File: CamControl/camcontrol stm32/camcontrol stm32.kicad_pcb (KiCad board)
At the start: 4 copper layers, 15.9 x 25.4 mm, 53 parts, among them J1 Power 1, J3 Power 1, J4 Power 1, J5 Conn_01x06, J6 Conn_01x02, J7 Power 1, J8 DNP, Q1 AO3401A, Q3 AO3401A, U1 BGS12WN6E6327, U2 BALFHB-WL-02D3, U3 STM32WLE4CCUx, U4 XC6206P332MR, U5 TPS25970LRPWR, U6 TPS25970LRPWR, U7 INA2180, Y1 32MHz

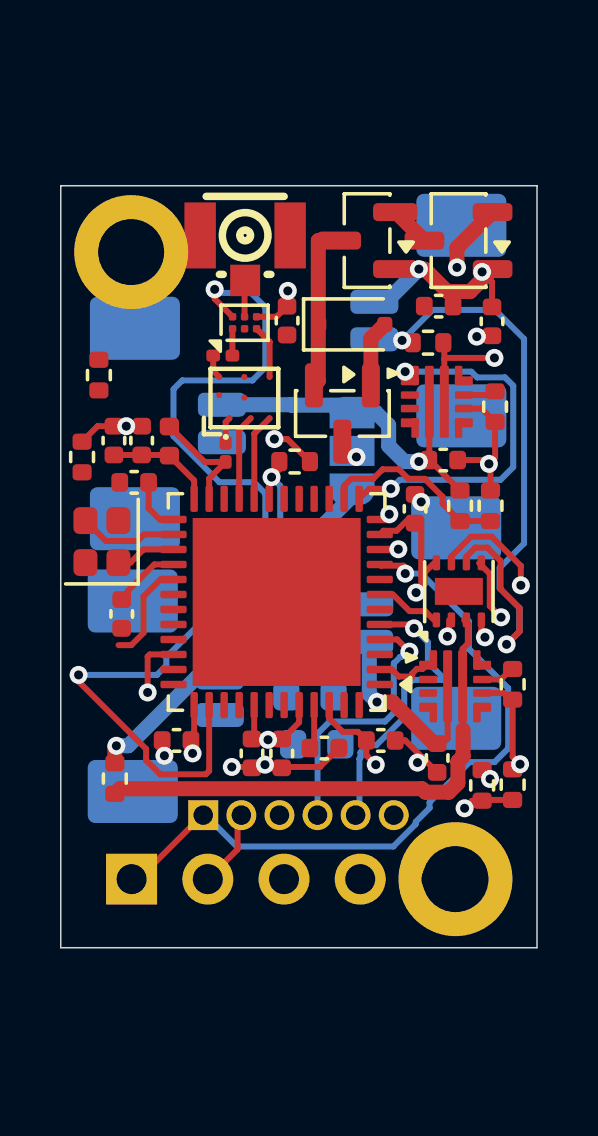
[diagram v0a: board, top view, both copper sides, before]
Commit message: final version?
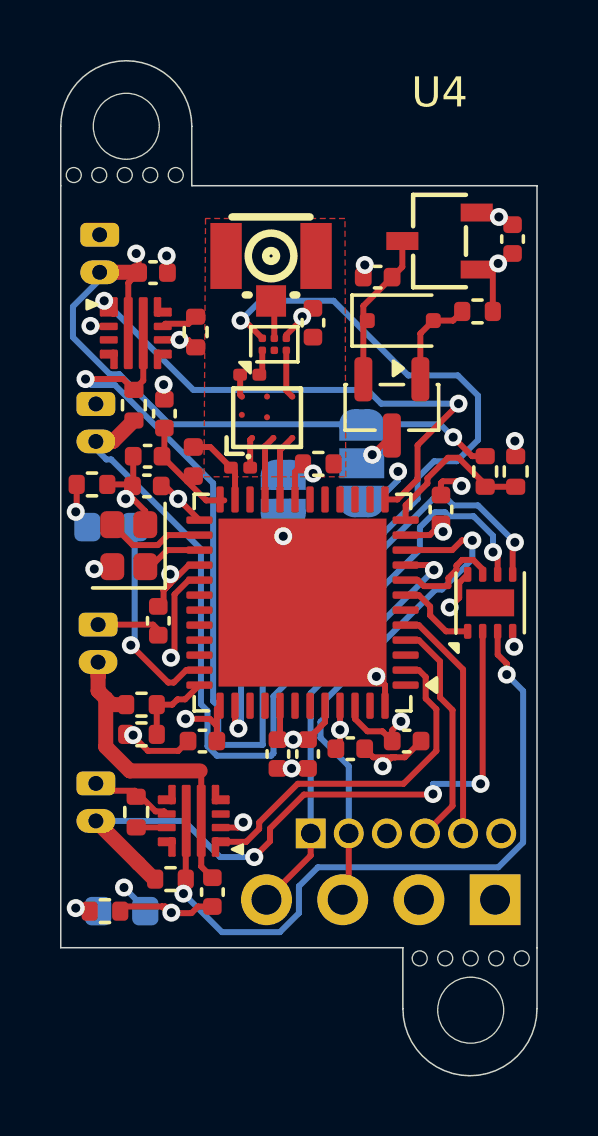
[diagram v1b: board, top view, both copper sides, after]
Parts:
- removed D4: D_Schottky, Diode_SMD:D_SOD-323F
- removed J8: DNP, Connector_PinHeader_2.54mm:PinHeader_1x05_P2.54mm_Vertical
- removed Q3: AO3401A, Package_TO_SOT_SMD:SOT-23
- added D3: D_Zener, Diode_SMD:D_SOD-323F, F.Cu at (170.3, 124.3)
- added J2: Conn_01x04, Connector_PinHeader_2.54mm:PinHeader_1x04_P2.54mm_Vertical, B.Cu at (173.4, 143.6)
- added R10: 51k, Resistor_SMD:R_0402_1005Metric, F.Cu at (172.8, 124.0)
- added REF**: BreakLine_5h_D0.5mm_P0.85mm, Panelization:BreakLine_5h_D0.5mm_P0.85mm, F.Cu at (161.1, 119.5)
- added REF**: BreakLine_5h_D0.5mm_P0.85mm, Panelization:BreakLine_5h_D0.5mm_P0.85mm, F.Cu at (172.6, 145.6)
- H1, H2: value MountingHole_Pad -> MountingHole; footprint MountingHole:MountingHole_2.2mm_M2_DIN965_Pad -> MountingHole:MountingHole_2.2mm_M2_DIN965; moved to B.Cu
- J1, J3, J4, J7: footprint Connector_Molex:Molex_PicoBlade_53261-0271_1x02-1MP_P1.25mm_Horizontal -> Connector_Molex:Molex_PicoBlade_53048-0210_1x02_P1.25mm_Horizontal
- U4: value XC6206P332MR -> DS8242; footprint Package_TO_SOT_SMD:SOT-23-3 -> .pretty:SOT-23-3_L2.9-W1.6-P1.90-LS2.8-BR
- moved H2 27.7 mm to (172.6, 147.3)
- moved H1 27.4 mm to (161.1, 117.9)
- moved R1 17.9 mm to (160.4, 144.0), turned to 0 degrees
- moved R6 13.3 mm to (161.5, 140.7), turned to 90 degrees
- moved R9 12.5 mm to (161.6, 138.1), turned to 180 degrees
- moved J3 12.0 mm to (160.1, 127.1)
- moved R8 11.7 mm to (161.6, 137.1), turned to 0 degrees
- moved C12 11.5 mm to (162.0, 122.7)
- moved J4 11.4 mm to (160.2, 134.5)
- moved U6 10.3 mm to (161.5, 124.8)
- moved R2 10.3 mm to (163.4, 124.7)
- moved R3 10.0 mm to (161.4, 127.2), turned to -90 degrees
- moved D2 9.97 mm to (160.6, 131.2), turned to 0 degrees
- moved U5 9.80 mm to (163.4, 141.0), turned to 180 degrees
- moved D1 9.52 mm to (161.0, 144.0), turned to 0 degrees
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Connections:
- Q1 pad 1: GND -> Net-(D3-A)
- Q1 pad 3: Net-(D4-K) -> Net-(JP1-C)
- U3 pad 12: /BATT SENSE A -> /BATT SENSE B
- U3 pad 14: /BATT SENSE B -> unconnected-(U3-PA6-Pad14)
- U3 pad 30: /LED INDICATION -> unconnected-(U3-PB0-Pad30)
- U3 pad 34: /CURRENT SENSE B -> unconnected-(U3-PA11-Pad34)
- U3 pad 35: unconnected-(U3-PA12-Pad35) -> /LED INDICATION
- U3 pad 36: unconnected-(U3-PA13-Pad36) -> /BATT SENSE A
- U3 pad 8: unconnected-(U3-PA1-Pad8) -> /CURRENT SENSE B
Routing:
- net /CURRENT SENSE B: track 28.7 -> 3.56 mm, vias 2 -> 0
- net /PWR B SENS: track 15.7 -> 34.7 mm
- net /PWR A: track 5.76 -> 22.8 mm, vias 2 -> 3
- net +12V: track 11.4 -> 22.1 mm, vias 1 -> 2
- net /PRWA EN: track 2.07 -> 12.1 mm
- net /CAM1 RX: track 23.9 -> 14.3 mm
- net /PWR B: track 20.7 -> 29.6 mm, vias 2 -> 1
- net +12VA: track 18.3 -> 26.5 mm, vias 2 -> 1
- net /CAM1 TX: track 24.6 -> 17.0 mm
- net /LED INDICATION: track 0.00 -> 6.96 mm, vias 0 -> 1
- net /VFBSMPS: track 4.95 -> 11.5 mm, vias 0 -> 2
- net /RF CTRL: track 32.4 -> 26.1 mm
- net /PWR A SENS: track 17.3 -> 23.5 mm, vias 0 -> 2
- net /PWRB EN: track 12.1 -> 17.7 mm
- net Net-(D4-K): track 5.58 -> 0.00 mm
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- added copper zone on F.Cu, net GND
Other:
- board size 15.9 x 25.4 mm -> 15.9 x 33.8 mm
- board text added: "- +"
- board text added: "A IN"
- board text added: "A OUT"
- board text added: "B A"
- board text added: "B IN"
- board text added: "B OUT"
- board text added: "GND TX RX GND TX RX"
- board text added: "THE THING AMAJIG"
